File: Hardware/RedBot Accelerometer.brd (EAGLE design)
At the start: 11.4 x 17.8 mm, 17 parts, among them U1 MMA8452Q, U2 MIC5205-3.3V, U3 PCA9306

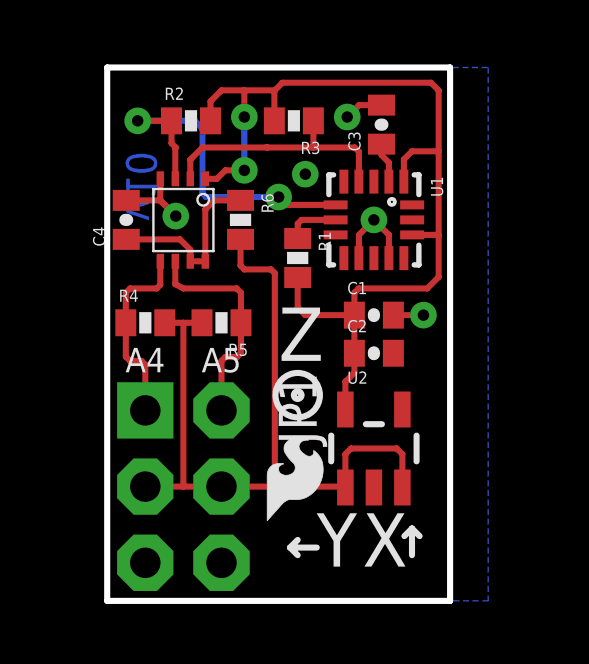
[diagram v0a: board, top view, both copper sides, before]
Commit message: Rev for v11 protos
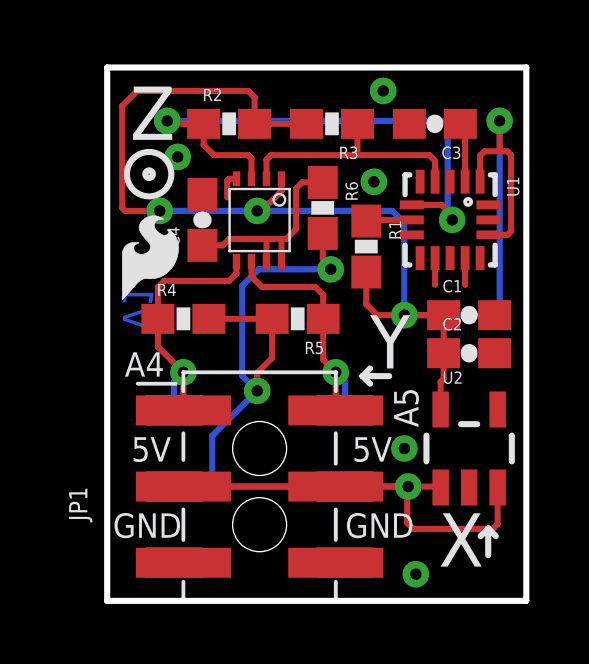
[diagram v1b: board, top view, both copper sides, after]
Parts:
- added JP2: (no value), SparkFun-Connectors:2X3_SMD
- C1, C2, C3, C4: device SparkFun-Capacitors:0402-CAP -> SparkFun-Capacitors:0603-CAP
- JP1: device SparkFun-Connectors:2X3-NS -> SparkFun-Connectors:2X3_SMT_POSTS
- R1, R2, R3, R4, R5, R6: device SparkFun-Resistors:0402-RES -> SparkFun-Resistors:0603-RES
- moved FRAME1 78.7 mm to (0.00, -12.7)
- moved LOGO1 8.81 mm to (0.51, 10.0)
- moved C1 3.17 mm to (12.1, 9.53)
- moved C2 3.17 mm to (12.1, 8.26)
- moved U2 3.17 mm to (12.1, 5.08)
- moved R6 2.77 mm to (7.18, 13.1)
- moved R5 2.54 mm to (6.35, 9.40)
- moved C4 2.54 mm to (3.17, 12.7)
- moved JP1 2.54 mm to (5.08, 3.81)
- moved U3 2.54 mm to (5.08, 12.7)
- moved LOGO2 2.54 mm to (11.4, 14.2)
- moved U1 2.54 mm to (11.4, 12.7)
- moved R1 2.32 mm to (8.64, 11.8)
- moved C3 1.78 mm to (10.9, 15.9), turned to 180 degrees
- moved R4 1.28 mm to (2.54, 9.40)
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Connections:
- net 5V: now also JP2.3, JP2.4
- net GND: now also JP2.5, JP2.6
- net SCL: now also JP2.1
- net SDA: now also JP2.2
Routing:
- net 3.3V: track 32.9 -> 47.8 mm, vias 2 -> 4
- net 5V: track 26.9 -> 38.7 mm, vias 0 -> 3
- net SDA1: track 12.1 -> 18.7 mm
- net GND: track 8.60 -> 2.66 mm
- net SDA: track 6.46 -> 9.07 mm, vias 0 -> 1
- net SCL: track 7.46 -> 8.58 mm, vias 0 -> 1
- net N$2: track 6.19 -> 7.19 mm
- net N$1: track 1.35 -> 2.17 mm
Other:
- board size 11.4 x 17.8 mm -> 14 x 17.8 mm
- board text added: "v11"
- board text removed: "v10"
